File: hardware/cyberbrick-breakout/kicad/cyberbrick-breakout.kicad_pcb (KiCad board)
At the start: 2 copper layers, 60 x 36 mm, 34 parts, among them J1 LX, J10 DL_LFT, J11 DL_RGT, J12 DL_DWN, J13 DR_UP, J14 DR_LFT, J15 DR_RGT, J16 DR_DWN, J17 SHL1, J18 SHL2, J19 SHR1, J2 LY, J20 SHR2, J21 START, J22 SEL, J23 HOTKEY, J24 COIN, J3 RX, J4 RY, J6A GPA, J6B GPB, J7 I2C, J8 PWR, J9 DL_UP, U1A ESP32-C3 top, U1B ESP32-C3 bot

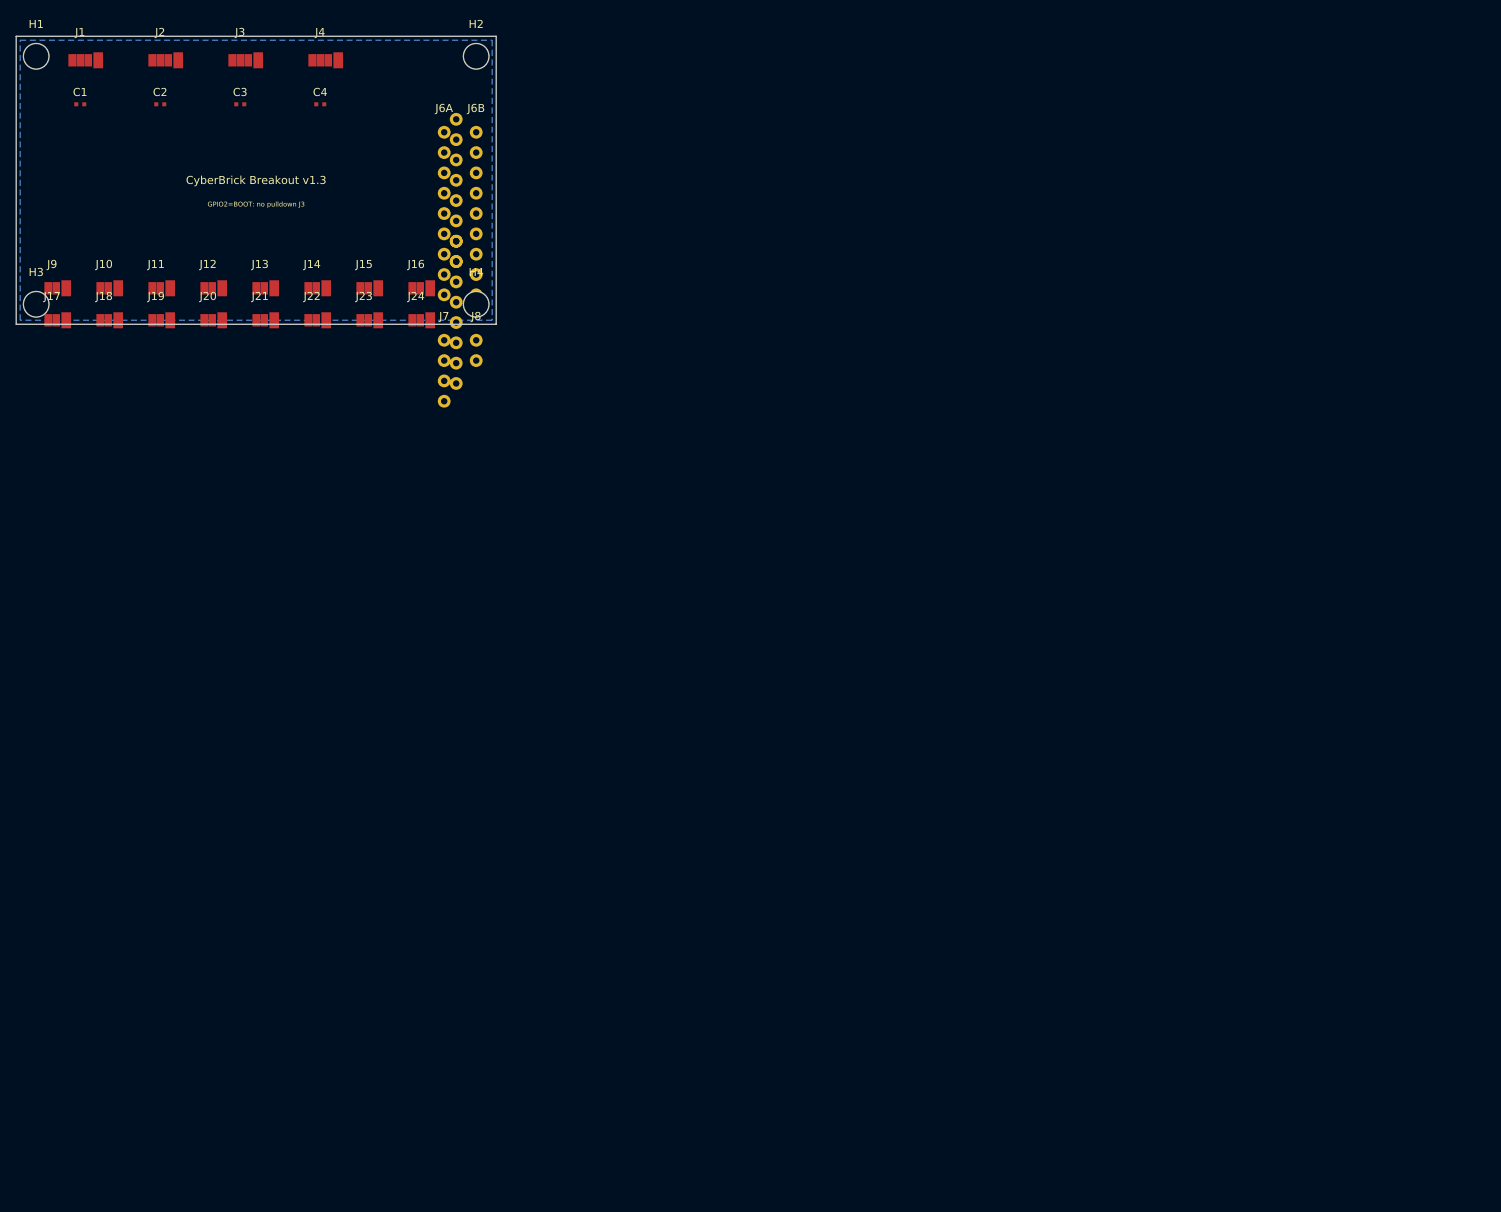
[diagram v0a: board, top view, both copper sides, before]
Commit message: latest layout
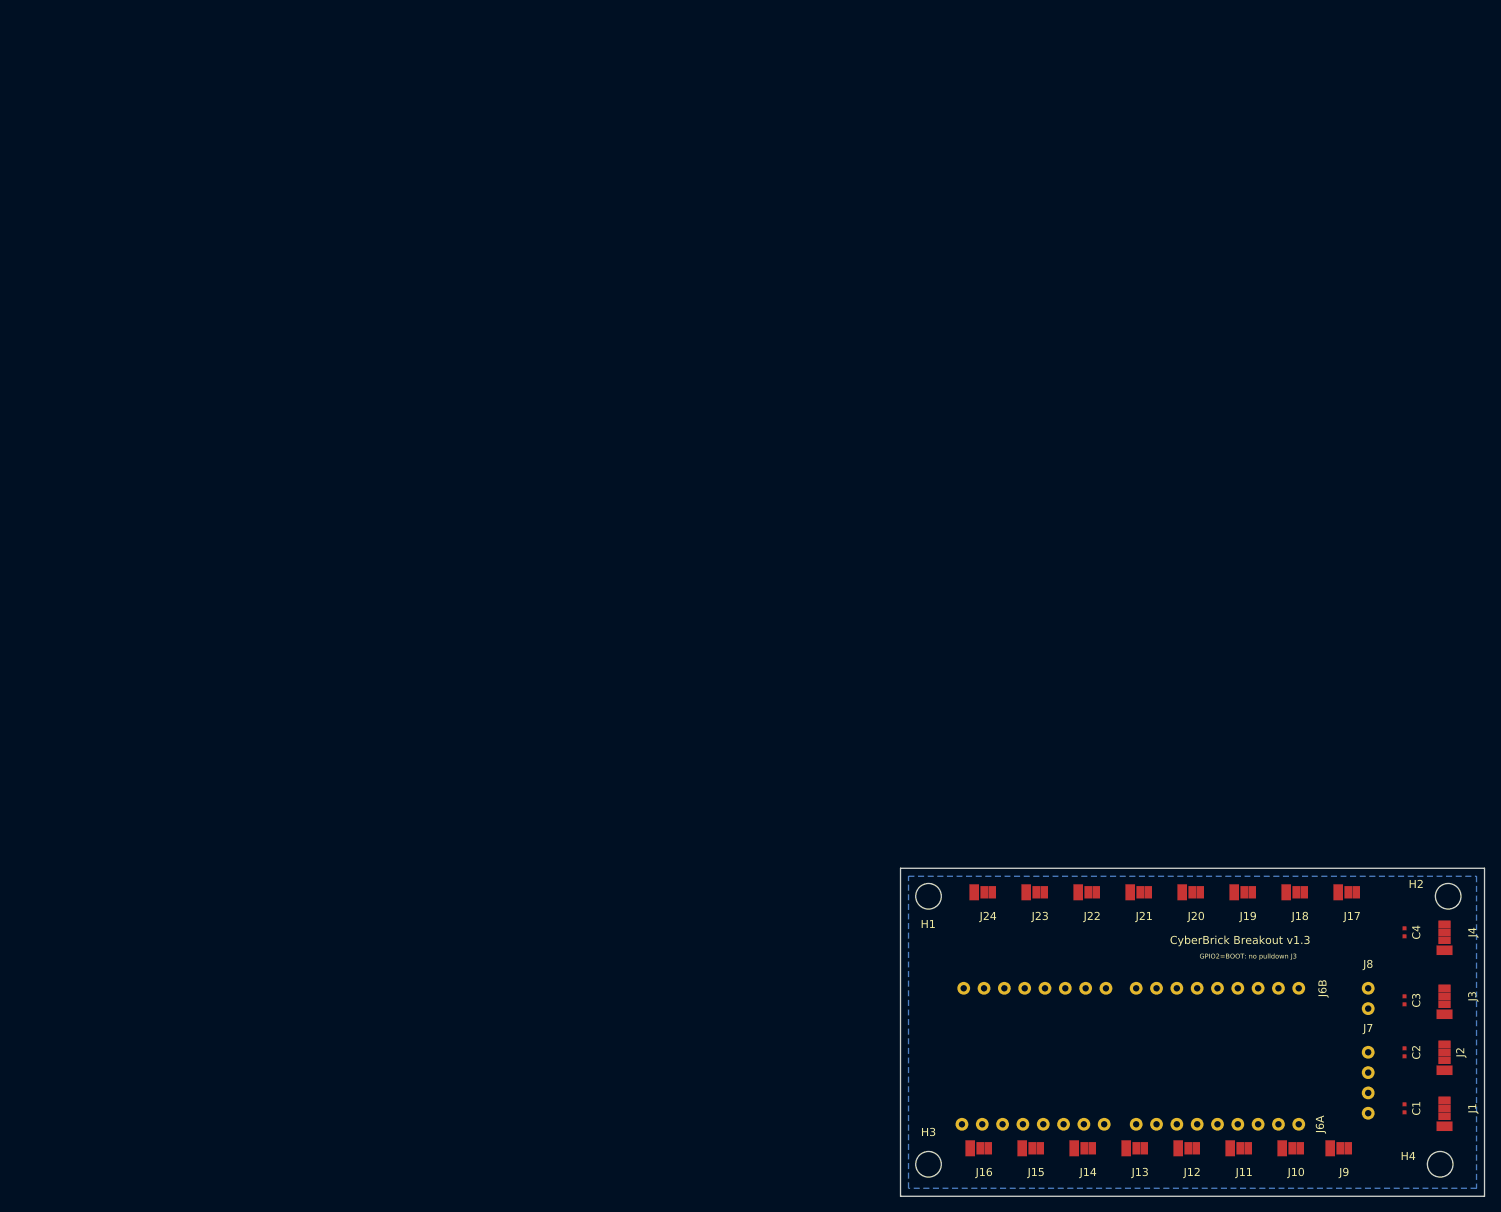
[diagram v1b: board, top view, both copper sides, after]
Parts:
- moved J1 215.0 mm to (178.5, 134.0), turned to -90 degrees
- moved C1 207.7 mm to (173.5, 134.0), turned to -90 degrees
- moved J2 202.9 mm to (178.5, 127.0), turned to -90 degrees
- moved C2 195.5 mm to (173.5, 127.0), turned to -90 degrees
- moved J9 194.0 mm to (166.0, 139.0), turned to 180 degrees
- moved J3 190.7 mm to (178.5, 120.0), turned to -90 degrees
- moved J10 183.7 mm to (160.0, 139.0), turned to 180 degrees
- moved C3 183.6 mm to (173.5, 120.5), turned to -90 degrees
- moved J4 177.9 mm to (178.5, 112.0), turned to -90 degrees
- moved J17 177.5 mm to (167.0, 107.0), turned to 180 degrees
- moved J11 173.4 mm to (153.5, 139.0), turned to 180 degrees
- moved C4 170.5 mm to (173.5, 112.0), turned to -90 degrees
- moved J18 165.7 mm to (160.5, 107.0), turned to 180 degrees
- moved J6A 163.7 mm to (160.3, 136.0), turned to -90 degrees
- moved J12 163.4 mm to (147.0, 139.0), turned to 180 degrees
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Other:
- board size 60 x 36 mm -> 73 x 41 mm
